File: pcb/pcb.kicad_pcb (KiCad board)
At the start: 4 copper layers, 107 parts, among them J1 Conn_02x10_Odd_Even, J2 Conn_02x03_Counter_Clockwise, Q1 BSS138, Q10 BSS138, Q11 BSS138, Q12 BSS138, Q2 BSS138, Q3 BSS138, Q4 BSS138, Q5 BSS138, Q6 BSS138, Q7 BSS138, Q8 BSS138, Q9 BSS138, SW1 SW_PUSHBUTTON, SW2 SW_PUSHBUTTON, SW3 SW_PUSHBUTTON, SW4 SW_PUSHBUTTON, U1 EFM32GG980, U2 ARDUINO_PYNQ_SHIELD, U3 IMU, U4 lidar, U5 ULTRASONIC-GPIO, U6 ULTRASONIC-GPIO, U7 ULTRASONIC-GPIO, Y1 Crystal_GND23

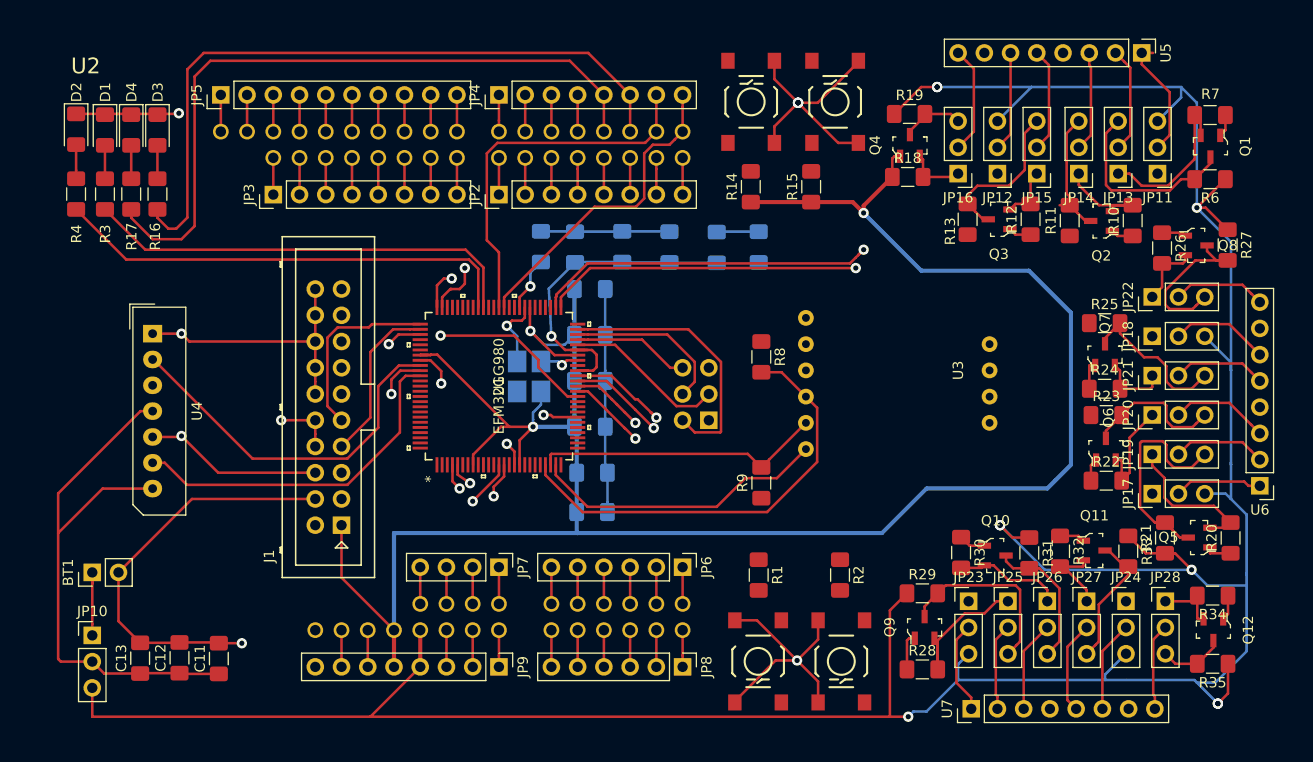
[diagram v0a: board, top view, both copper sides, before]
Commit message: Think it is somewhat finished
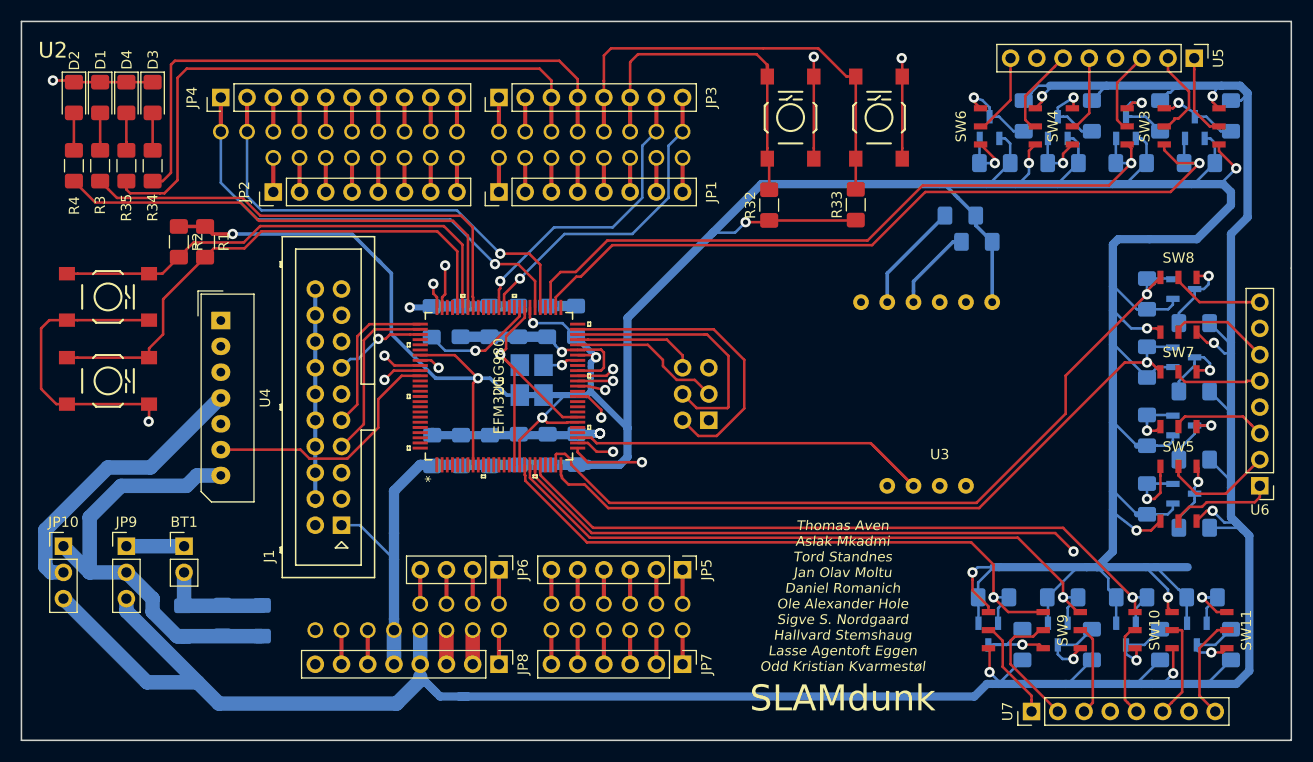
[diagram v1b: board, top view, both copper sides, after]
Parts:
- removed JP11, JP12, JP13, JP14, JP15, JP16, JP17, JP18, JP19, JP20, JP21, JP22, JP23, JP24, JP25, JP26, JP27, JP28: Jumper_NC_Dual, Connector_PinHeader_2.54mm:PinHeader_1x03_P2.54mm_Vertical
- added JP1: M08, Connector_PinHeader_2.54mm:PinHeader_1x08_P2.54mm_Vertical, F.Cu at (101.6, 59.2)
- added SW10: SW_2xSPDT, localization-footprints:CAS-D20TB, F.Cu at (160.5, 101.6)
- added SW11: SW_2xSPDT, localization-footprints:CAS-D20TB, F.Cu at (169.4, 101.6)
- added SW12: SW_PUSHBUTTON, myfootprint:SW_PUSHBUTTON_SMD, F.Cu at (129.8, 52.0)
- added SW13: SW_PUSHBUTTON, myfootprint:SW_PUSHBUTTON_SMD, F.Cu at (138.4, 52.0)
- added SW5: SW_2xSPDT, localization-footprints:CAS-D20TB, F.Cu at (167.4, 88.4)
- added SW6: SW_2xSPDT, localization-footprints:CAS-D20TB, F.Cu at (150.9, 52.8)
- added SW7: SW_2xSPDT, localization-footprints:CAS-D20TB, F.Cu at (167.4, 79.2)
- added SW8: SW_2xSPDT, localization-footprints:CAS-D20TB, F.Cu at (167.4, 70.1)
- added SW9: SW_2xSPDT, localization-footprints:CAS-D20TB, F.Cu at (151.6, 101.6)
- C11, C12, C13, Q1, Q10, Q11, Q12, Q2, Q3, Q4, Q5, Q6, Q7, Q8, Q9, R10, R11, R12, R13, R18, R19, R20, R21, R22, R23, R24, R25, R26, R27, R28, R29, R30, R31: moved to B.Cu
- JP4: value M08 -> M10; footprint Connector_PinHeader_2.54mm:PinHeader_1x08_P2.54mm_Vertical -> Connector_PinHeader_2.54mm:PinHeader_1x10_P2.54mm_Vertical
- JP5: value M10 -> M06; footprint Connector_PinHeader_2.54mm:PinHeader_1x10_P2.54mm_Vertical -> Connector_PinHeader_2.54mm:PinHeader_1x06_P2.54mm_Vertical
- JP6: value M06 -> M04; footprint Connector_PinHeader_2.54mm:PinHeader_1x06_P2.54mm_Vertical -> Connector_PinHeader_2.54mm:PinHeader_1x04_P2.54mm_Vertical
- JP7: value M04 -> M06; footprint Connector_PinHeader_2.54mm:PinHeader_1x04_P2.54mm_Vertical -> Connector_PinHeader_2.54mm:PinHeader_1x06_P2.54mm_Vertical
- JP8: value M06 -> M08; footprint Connector_PinHeader_2.54mm:PinHeader_1x06_P2.54mm_Vertical -> Connector_PinHeader_2.54mm:PinHeader_1x08_P2.54mm_Vertical
- JP9: value M08 -> Jumper_NC_Dual; footprint Connector_PinHeader_2.54mm:PinHeader_1x08_P2.54mm_Vertical -> Connector_PinHeader_2.54mm:PinHeader_1x03_P2.54mm_Vertical
- R14, R15, R16, R17: value R -> 10k; moved to B.Cu
- R32, R33, R34, R35: value 10k -> R
- R6: value 10k -> 2.2k; moved to B.Cu
- R7: value 10k -> 4.7k; moved to B.Cu
- R8: value 2.2k -> 10k; moved to B.Cu
- R9: value 4.7k -> 10k; moved to B.Cu
- SW3, SW4: value SW_PUSHBUTTON -> SW_2xSPDT; footprint myfootprint:SW_PUSHBUTTON_SMD -> localization-footprints:CAS-D20TB
- moved R35 115.7 mm to (65.5, 56.6), turned to 90 degrees
- moved R34 110.7 mm to (68.1, 56.6), turned to 90 degrees
- moved R17 93.3 mm to (159.0, 51.8), turned to 270 degrees
- moved R16 87.7 mm to (156.2, 56.4), turned to 180 degrees
- moved SW2 79.3 mm to (63.8, 69.3), turned to 0 degrees
- moved R2 71.7 mm to (70.6, 64.0)
- moved SW1 68.5 mm to (63.8, 77.5), turned to 0 degrees
- moved JP5 64.1 mm to (119.4, 95.8), turned to 270 degrees
- moved R1 62.6 mm to (73.2, 64.0)
- moved R9 57.7 mm to (172.5, 51.8), turned to 270 degrees
- moved R8 46.4 mm to (169.4, 56.4), turned to 180 degrees
- moved R15 45.5 mm to (168.9, 85.1), turned to 180 degrees
- moved R14 45.0 mm to (164.3, 82.3)
- moved R32 43.8 mm to (127.8, 60.5), turned to 90 degrees
- moved R21 43.1 mm to (152.4, 51.8), turned to 270 degrees
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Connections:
- JP10 pad 1: Net-(BT1-Pad1) -> Net-(C11-Pad1)
- JP10 pad 2: Net-(C11-Pad1) -> Net-(JP10-Pad2)
- JP3 pad 3: Net-(JP3-Pad3) -> /PYNQ-DEBUG/LED_2
- JP3 pad 4: Net-(JP3-Pad4) -> /PYNQ-DEBUG/LED_1
- JP3 pad 5: Net-(JP3-Pad5) -> /PYNQ-DEBUG/SW_2
- JP3 pad 6: Net-(JP3-Pad6) -> /PYNQ-DEBUG/SW_1
- JP3 pad 7: Net-(JP3-Pad7) -> /PYNQ_TX
- JP3 pad 8: Net-(JP3-Pad8) -> /PYNQ_RX
- JP4 pad 1: Net-(JP4-Pad1) -> /PYNQ_SCL
- JP4 pad 2: Net-(JP4-Pad2) -> /PYNQ_SDA
- JP4 pad 3: /PYNQ-DEBUG/SW_2 -> Net-(JP4-Pad3)
- JP4 pad 4: /PYNQ-DEBUG/SW_1 -> Net-(JP4-Pad4)
- JP4 pad 5: /PYNQ-DEBUG/LED_2 -> Net-(JP4-Pad5)
- JP4 pad 6: /PYNQ-DEBUG/LED_1 -> Net-(JP4-Pad6)
- JP4 pad 7: /PYNQ_TX -> Net-(JP4-Pad7)
- JP4 pad 8: /PYNQ_RX -> Net-(JP4-Pad8)
- JP5 pad 1: /PYNQ_SCL -> Net-(JP5-Pad1)
- JP5 pad 2: /PYNQ_SDA -> Net-(JP5-Pad2)
- JP8 pad 2: Net-(JP8-Pad2) -> GND
- JP8 pad 3: Net-(JP8-Pad3) -> GND
- JP8 pad 4: Net-(JP8-Pad4) -> VCC
- JP8 pad 5: Net-(JP8-Pad5) -> +3V3
- JP9 pad 1: Net-(JP9-Pad1) -> Net-(BT1-Pad1)
- JP9 pad 2: GND -> Net-(C11-Pad1)
- JP9 pad 3: GND -> VCC
- Q1 pad 2: /PD5 -> /PD6_A1
- Q1 pad 3: Net-(JP13-Pad3) -> Net-(Q1-Pad3)
- Q10 pad 2: /PB5 -> /PC1_B2
- Q10 pad 3: Net-(JP26-Pad3) -> Net-(Q10-Pad3)
- Q11 pad 2: /PA4 -> /PC3_BRX
- Q11 pad 3: Net-(JP27-Pad3) -> Net-(Q11-Pad3)
- Q12 pad 2: /PA3 -> /PC2_BTX
- Q12 pad 3: Net-(JP28-Pad3) -> Net-(Q12-Pad3)
- Q2 pad 2: /PD6 -> /PA7_C1
- Q3 pad 2: /PF11 -> /PD7_A2
- Q3 pad 3: Net-(JP15-Pad3) -> Net-(Q3-Pad3)
- Q4 pad 2: /PF10 -> /PA8_C2
- Q4 pad 3: Net-(JP16-Pad3) -> Net-(Q4-Pad3)
- Q5 pad 2: /PB11 -> /PF11_ARX
- Q5 pad 3: Net-(JP19-Pad3) -> Net-(Q5-Pad3)
- Q6 pad 2: /PB12 -> /PB8_CRX
- Q6 pad 3: Net-(JP20-Pad3) -> Net-(Q6-Pad3)
- Q7 pad 2: /PB10 -> /PF10_ATX
- Q7 pad 3: Net-(JP21-Pad3) -> Net-(Q7-Pad3)
- Q8 pad 2: /PB9 -> /PB7_CTX
- Q8 pad 3: Net-(JP22-Pad3) -> Net-(Q8-Pad3)
- Q9 pad 2: /PB4 -> /PC0_B1
- Q9 pad 3: Net-(JP25-Pad3) -> Net-(Q9-Pad3)
- R1 pad 2: /PC1 -> /EFM_DEBUG/SW_1
- R10 pad 2: /PD6 -> /PA7_C1
- R12 pad 2: /PF11 -> /PD7_A2
- R13 pad 2: Net-(JP15-Pad3) -> Net-(Q3-Pad3)
- R14 pad 2: /PYNQ-DEBUG/SW_1 -> /PA8_C2
- R15 pad 1: +3V3 -> VCC
- R15 pad 2: /PYNQ-DEBUG/SW_2 -> Net-(Q4-Pad3)
- R16 pad 1: /PYNQ-DEBUG/LED_1 -> +3V3
- R16 pad 2: Net-(D3-Pad2) -> /PF11_ARX
- R17 pad 1: /PYNQ-DEBUG/LED_2 -> VCC
- R17 pad 2: Net-(D4-Pad2) -> Net-(Q5-Pad3)
- R18 pad 2: /PF10 -> /PB8_CRX
- R19 pad 2: Net-(JP16-Pad3) -> Net-(Q6-Pad3)
- R2 pad 2: /PC0 -> /EFM_DEBUG/SW_2
- R20 pad 2: /PB11 -> /PF10_ATX
- R21 pad 2: Net-(JP19-Pad3) -> Net-(Q7-Pad3)
- R22 pad 2: /PB12 -> /PB7_CTX
- R23 pad 2: Net-(JP20-Pad3) -> Net-(Q8-Pad3)
- R24 pad 2: /PB10 -> /PC0_B1
- R25 pad 2: Net-(JP21-Pad3) -> Net-(Q9-Pad3)
- R26 pad 2: /PB9 -> /PC1_B2
- R27 pad 2: Net-(JP22-Pad3) -> Net-(Q10-Pad3)
- R28 pad 2: /PB4 -> /PC3_BRX
- R29 pad 2: Net-(JP25-Pad3) -> Net-(Q11-Pad3)
- R30 pad 2: /PB5 -> /PC2_BTX
- R31 pad 2: Net-(JP26-Pad3) -> Net-(Q12-Pad3)
- R32 pad 2: /PA4 -> /PYNQ-DEBUG/SW_1
- R33 pad 1: VCC -> +3V3
- R33 pad 2: Net-(JP27-Pad3) -> /PYNQ-DEBUG/SW_2
- R34 pad 1: +3V3 -> /PYNQ-DEBUG/LED_1
- R34 pad 2: /PA3 -> Net-(D3-Pad2)
- R35 pad 1: VCC -> /PYNQ-DEBUG/LED_2
- R35 pad 2: Net-(JP28-Pad3) -> Net-(D4-Pad2)
- R6 pad 1: VCC -> +3V3
- R6 pad 2: Net-(JP13-Pad3) -> /PB11_IMU_SDA
- R7 pad 2: /PD5 -> /PB12_IMU_SCL
- R8 pad 2: /IMU/SDA -> /PD6_A1
- R9 pad 1: +3V3 -> VCC
- R9 pad 2: /IMU/SCL -> Net-(Q1-Pad3)
- SW1 pad 1: /PC1 -> /EFM_DEBUG/SW_1
- SW2 pad 1: /PC0 -> /EFM_DEBUG/SW_2
- SW3 pad 1: /PYNQ-DEBUG/SW_1 -> VCC
- SW3 pad 2: GND -> Net-(SW3-Pad2)
- SW4 pad 1: /PYNQ-DEBUG/SW_2 -> Net-(Q3-Pad3)
- SW4 pad 2: GND -> Net-(SW4-Pad2)
- U1 pad 13: /PB4 -> Net-(U1-Pad13)
- U1 pad 14: /PB5 -> Net-(U1-Pad14)
- U1 pad 18: /PC0 -> /PC0_B1
- U1 pad 19: /PC1 -> /PC1_B2
- U1 pad 20: Net-(U1-Pad20) -> /PC2_BTX
- U1 pad 21: Net-(U1-Pad21) -> /PC3_BRX
- U1 pad 22: /IMU/SDA -> Net-(U1-Pad22)
- U1 pad 23: /IMU/SCL -> Net-(U1-Pad23)
- U1 pad 24: /IMU/RST -> /PB7_CTX
- U1 pad 25: Net-(U1-Pad25) -> /PB8_CRX
- U1 pad 26: Net-(U1-Pad26) -> /PA7_C1
- U1 pad 27: Net-(U1-Pad27) -> /PA8_C2
- U1 pad 28: Net-(U1-Pad28) -> /PA9_IMU_INT
- U1 pad 37: /PB9 -> Net-(U1-Pad37)
- U1 pad 38: /PB10 -> /PB10_IMU_RST
- U1 pad 39: /PB11 -> /PB11_IMU_SDA
- U1 pad 4: /PA3 -> Net-(U1-Pad4)
- U1 pad 40: /PB12 -> /PB12_IMU_SCL
- U1 pad 5: /PA4 -> Net-(U1-Pad5)
- U1 pad 51: /PD5 -> Net-(U1-Pad51)
- U1 pad 52: /PD6 -> /PD6_A1
- U1 pad 53: Net-(U1-Pad53) -> /PD7_A2
- U1 pad 66: /EFM_DEBUG/LED_1 -> Net-(U1-Pad66)
- U1 pad 67: /EFM_DEBUG/LED_2 -> Net-(U1-Pad67)
- U1 pad 68: Net-(U1-Pad68) -> /EFM_DEBUG/LED_1
- U1 pad 69: Net-(U1-Pad69) -> /EFM_DEBUG/LED_2
- U1 pad 70: Net-(U1-Pad70) -> /EFM_DEBUG/SW_2
- U1 pad 71: Net-(U1-Pad71) -> /EFM_DEBUG/SW_1
- U1 pad 74: /PF10 -> /PF10_ATX
- U1 pad 75: /PF11 -> /PF11_ARX
- U2 pad 10: Net-(JP5-Pad8) -> Net-(JP4-Pad8)
- U2 pad 11: Net-(JP5-Pad7) -> Net-(JP4-Pad7)
- U2 pad 12: Net-(JP5-Pad6) -> Net-(JP4-Pad6)
- U2 pad 13: Net-(JP5-Pad5) -> Net-(JP4-Pad5)
- U2 pad 2: /PYNQ-DEBUG/LED_1 -> /PYNQ-DEBUG/SW_1
- U2 pad 26: Net-(JP2-Pad8) -> Net-(JP1-Pad8)
- U2 pad 27: Net-(JP2-Pad7) -> Net-(JP1-Pad7)
- U2 pad 28: Net-(JP2-Pad6) -> Net-(JP1-Pad6)
- U2 pad 29: Net-(JP2-Pad5) -> Net-(JP1-Pad5)
- U2 pad 3: /PYNQ-DEBUG/LED_2 -> /PYNQ-DEBUG/SW_2
- U2 pad 30: Net-(JP2-Pad4) -> Net-(JP1-Pad4)
- U2 pad 31: Net-(JP2-Pad3) -> Net-(JP1-Pad3)
- U2 pad 32: Net-(JP2-Pad2) -> Net-(JP1-Pad2)
- U2 pad 33: Net-(JP2-Pad1) -> Net-(JP1-Pad1)
- U2 pad 34: Net-(JP3-Pad8) -> Net-(JP2-Pad8)
- U2 pad 35: Net-(JP3-Pad7) -> Net-(JP2-Pad7)
- U2 pad 36: Net-(JP3-Pad6) -> Net-(JP2-Pad6)
- U2 pad 37: Net-(JP3-Pad5) -> Net-(JP2-Pad5)
- U2 pad 38: Net-(JP3-Pad4) -> Net-(JP2-Pad4)
- U2 pad 39: Net-(JP3-Pad3) -> Net-(JP2-Pad3)
- U2 pad 4: /PYNQ-DEBUG/SW_1 -> /PYNQ-DEBUG/LED_1
- U2 pad 40: Net-(JP3-Pad2) -> Net-(JP2-Pad2)
- U2 pad 41: Net-(JP3-Pad1) -> Net-(JP2-Pad1)
- U2 pad 5: /PYNQ-DEBUG/SW_2 -> /PYNQ-DEBUG/LED_2
- U2 pad 6: Net-(JP4-Pad2) -> Net-(JP3-Pad2)
- U2 pad 7: Net-(JP4-Pad1) -> Net-(JP3-Pad1)
- U2 pad 8: Net-(JP5-Pad10) -> Net-(JP4-Pad10)
- U2 pad 9: Net-(JP5-Pad9) -> Net-(JP4-Pad9)
- U2 pad A0: Net-(JP8-Pad6) -> Net-(JP7-Pad6)
- U2 pad A1: Net-(JP8-Pad5) -> Net-(JP7-Pad5)
- U2 pad A10: Net-(JP6-Pad2) -> Net-(JP5-Pad2)
- U2 pad A11: Net-(JP6-Pad1) -> Net-(JP5-Pad1)
- U2 pad A2: Net-(JP8-Pad4) -> Net-(JP7-Pad4)
- U2 pad A3: Net-(JP8-Pad3) -> Net-(JP7-Pad3)
- U2 pad A4: Net-(JP8-Pad2) -> Net-(JP7-Pad2)
- U2 pad A5: Net-(JP8-Pad1) -> Net-(JP7-Pad1)
- U2 pad A6: Net-(JP6-Pad6) -> Net-(JP5-Pad6)
- U2 pad A7: Net-(JP6-Pad5) -> Net-(JP5-Pad5)
- U2 pad A8: Net-(JP6-Pad4) -> Net-(JP5-Pad4)
- U2 pad A9: Net-(JP6-Pad3) -> Net-(JP5-Pad3)
- U2 pad A_R: Net-(JP5-Pad3) -> Net-(JP4-Pad3)
- U2 pad G: Net-(JP5-Pad4) -> Net-(JP4-Pad4)
- U2 pad IO_R: Net-(JP9-Pad7) -> Net-(JP8-Pad7)
- U2 pad RST: Net-(JP9-Pad6) -> Net-(JP8-Pad6)
- U2 pad VIN: Net-(JP9-Pad1) -> Net-(JP8-Pad1)
- U2 pad V_N: Net-(JP7-Pad3) -> Net-(JP6-Pad3)
- U2 pad V_P: Net-(JP7-Pad4) -> Net-(JP6-Pad4)
- U2 pad XGND: Net-(JP7-Pad2) -> Net-(JP6-Pad2)
- U2 pad XV_R: Net-(JP7-Pad1) -> Net-(JP6-Pad1)
- U3 pad 1: /IMU/RST -> /PB10_IMU_RST
- U3 pad 2: /IMU/SCL -> /PB12_IMU_SCL
- U3 pad 3: /IMU/SDA -> /PB11_IMU_SDA
- U3 pad 9: /IMU/INT -> /PA9_IMU_INT
- U4 pad 4: Net-(C11-Pad1) -> Net-(JP10-Pad2)
- U5 pad 1: Net-(JP11-Pad2) -> Net-(SW3-Pad2)
- U5 pad 2: Net-(JP13-Pad2) -> Net-(SW3-Pad5)
- U5 pad 3: Net-(JP14-Pad2) -> Net-(SW4-Pad2)
- U5 pad 5: Net-(JP15-Pad2) -> Net-(SW4-Pad5)
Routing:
- net +3V3: track 247.8 -> 435.4 mm, vias 3 -> 12
- net /PA3: track 83.1 -> 0.00 mm, vias 1 -> 0
- net /PA4: track 78.2 -> 0.00 mm, vias 1 -> 0
- net /PC2_BTX: track 0.00 -> 78.0 mm, vias 0 -> 2
- net /PB7_CTX: track 0.00 -> 77.2 mm, vias 0 -> 1
- net /PD6_A1: track 0.00 -> 77.1 mm, vias 0 -> 1
- net /PD5: track 76.7 -> 0.00 mm, vias 1 -> 0
- net GND: track 232.9 -> 156.9 mm, vias 13 -> 10
- net /PB9: track 74.8 -> 0.00 mm, vias 1 -> 0
- net /PB4: track 74.7 -> 0.00 mm, vias 1 -> 0
- net /PF11_ARX: track 0.00 -> 74.3 mm, vias 0 -> 2
- net /PB11: track 73.2 -> 0.00 mm, vias 1 -> 0
- net /PB5: track 72.4 -> 0.00 mm, vias 1 -> 0
- net /PB8_CRX: track 0.00 -> 71.4 mm, vias 0 -> 1
- net /PF11: track 70.1 -> 0.00 mm, vias 1 -> 0
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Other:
- board outline added: 122.9 x 69.6 mm
- board text added: "SLAMdunk"
- board text added: "Thomas Aven Aslak Mkadmi Tord Standnes Jan Olav Moltu Daniel Romanich Ole Alexander Hole Sigve S. Nordgaard Hallvard Stemshaug Lasse Agentoft Eggen Odd Kristian Kvarmestøl"
